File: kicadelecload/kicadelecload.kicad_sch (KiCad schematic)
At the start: 9 parts, among them Q1 IRF540N, Q2 IRF540N, Q3 IRF540N, Q4 IRF540N, U1 ESP32-S2-DEVKITC-1, U2 LM358, U3 TL431D

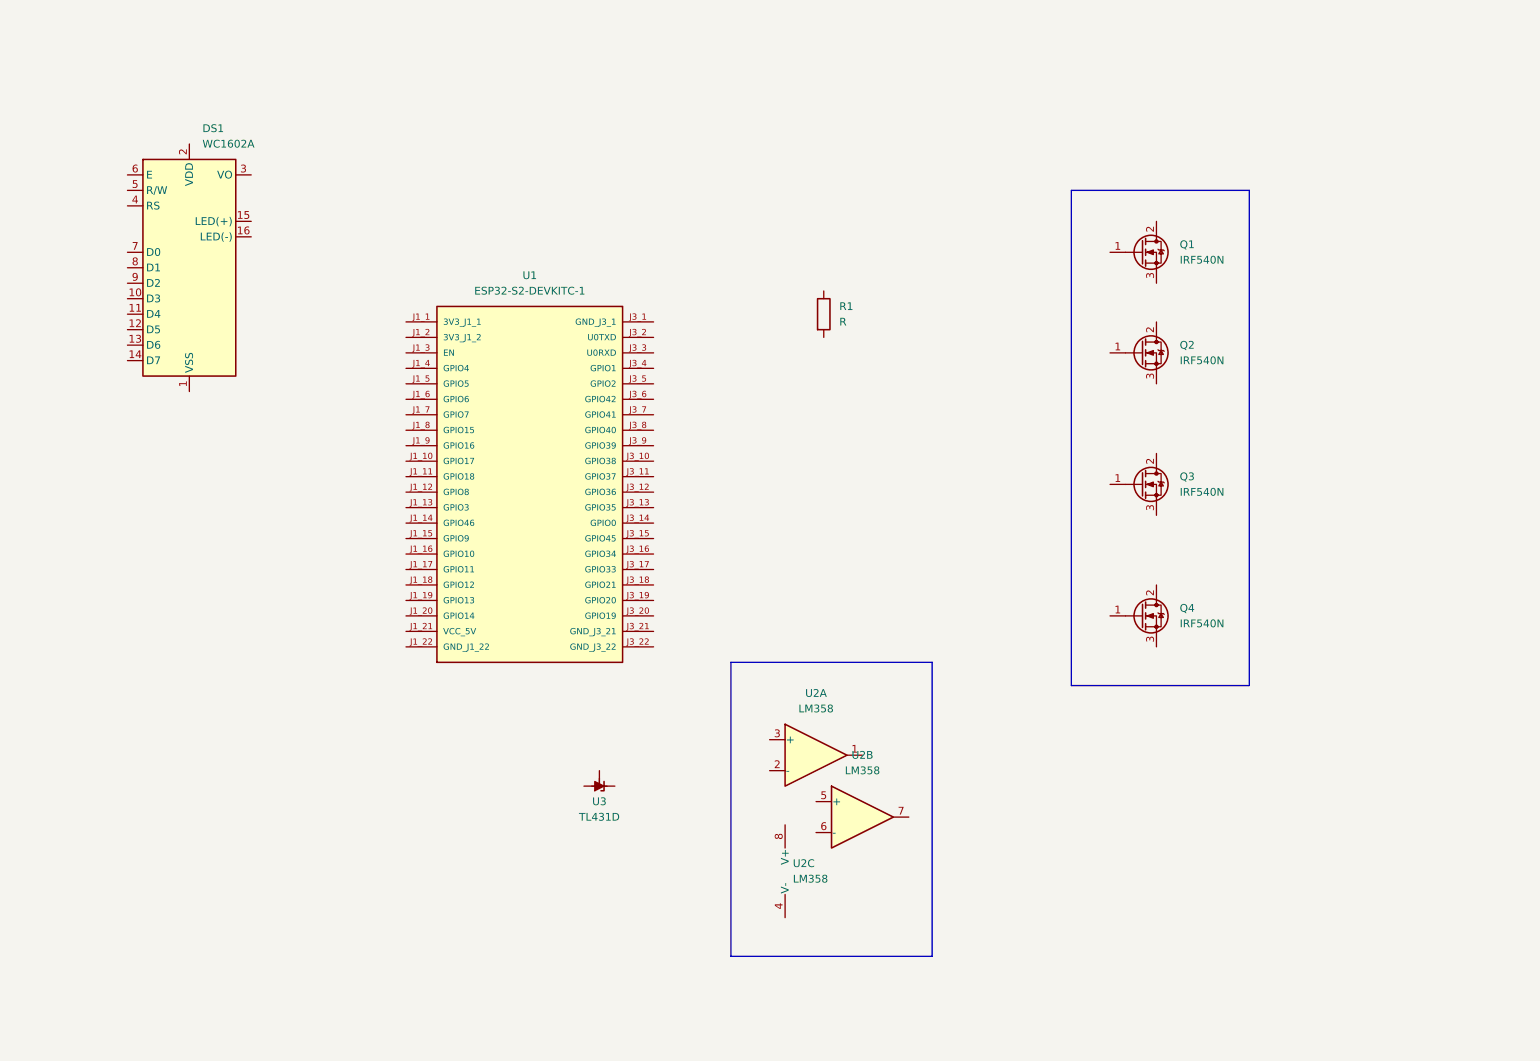
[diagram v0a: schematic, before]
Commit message: schéma electrique V1 commit 1
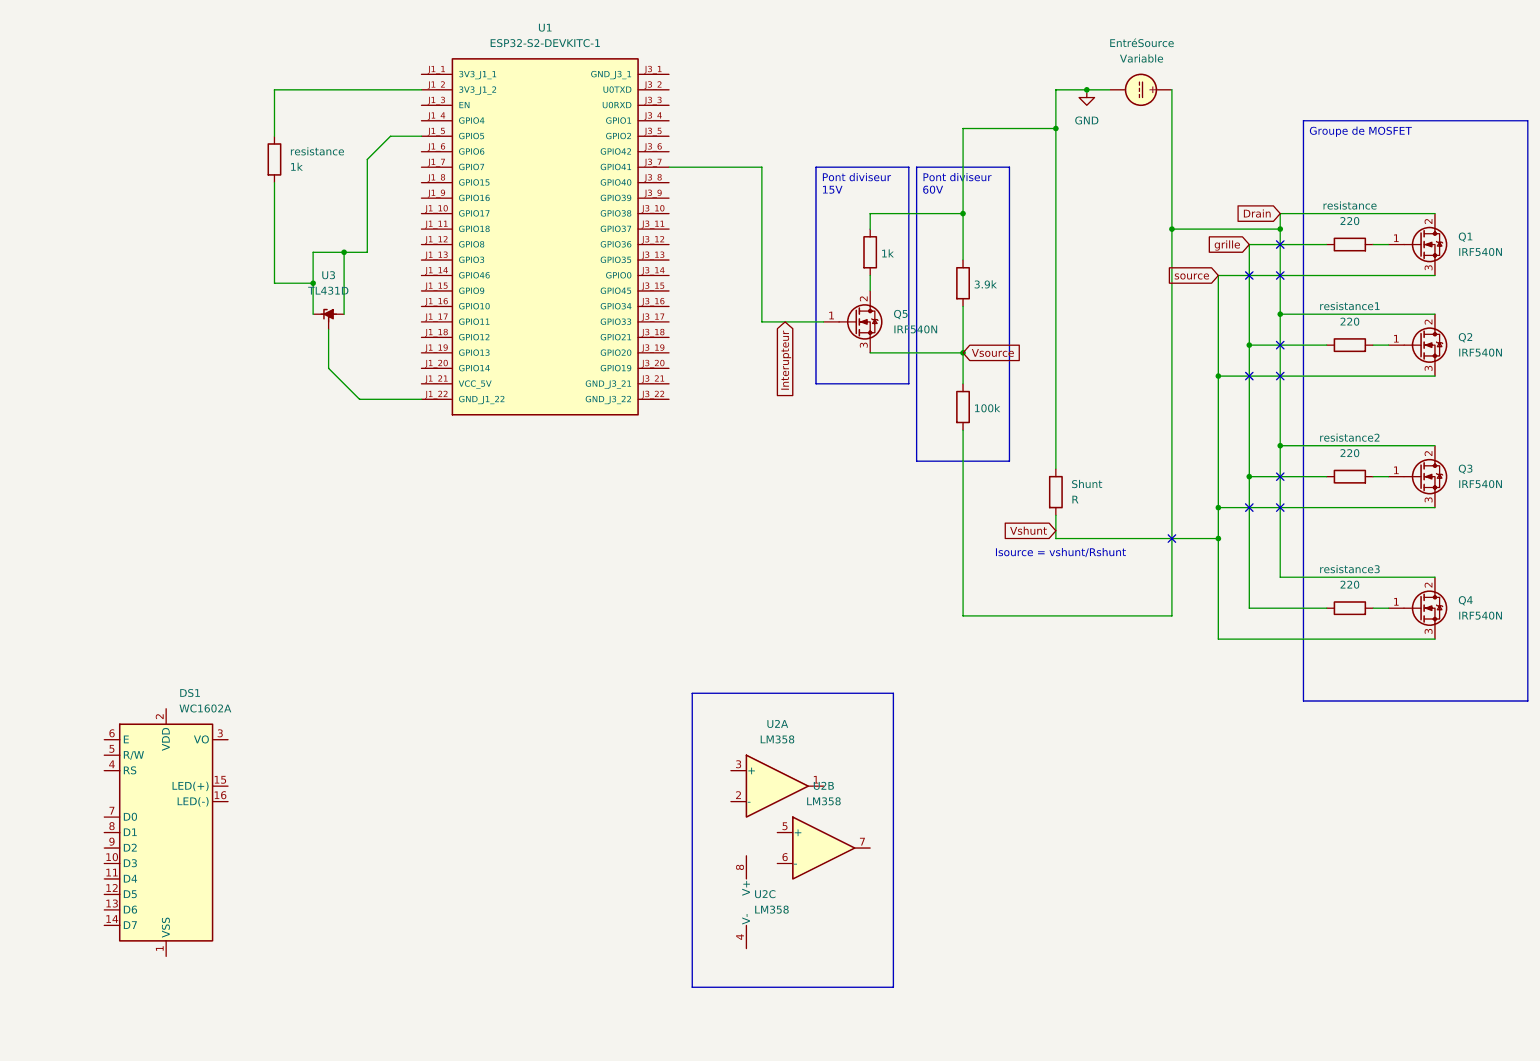
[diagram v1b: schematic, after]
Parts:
- added EntréSource: Variable, symbol Simulation_SPICE:VDC
- added Q5: IRF540N, Package_TO_SOT_THT:TO-220-3_Vertical, symbol Transistor_FET:IRF540N
- added resistance, resistance5: 1k, symbol Device:R
- added resistance, resistance1, resistance2, resistance3: 220, symbol Device:R
- added resistance4: 3.9k, symbol Device:R
- added resistance7: 100k, symbol Device:R
- renumbered R1 to Shunt
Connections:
- net at Q2.1 (G): now also resistance1.2
- net Drain: now reaches Q2.2 (D)
- net Drain: now also Q1.2 (D), Q3.2 (D), Q4.2 (D), EntréSource.1, resistance7.2
- net Vshunt: now reaches Q2.3 (S)
- net Vshunt: now also Q1.3 (S), Q3.3 (S), Q4.3 (S), Shunt.2
- net GND: now reaches Shunt.1
- net GND: now also EntréSource.2, resistance4.1, resistance5.1
- net at Q1.1 (G): now also resistance.2
- net at Q4.1 (G): now also resistance3.2
- net at Q3.1 (G): now also resistance2.2
- net at U3.1 (K): now also U1.J1_5 (GPIO5), U3.2 (A), U3.3 (A), U3.6 (A), U3.7 (A), resistance.2
- net at U3.8 (REF): now also U1.J1_22 (GND_J1_22)
- net at U1.J1_2 (3V3_J1_2): now also resistance.1
- net Interupteur: now reaches U1.J3_7 (GPIO41)
- net Interupteur: now also Q5.1 (G)
- new net: Q5.2 (D), resistance5.2
- new net Vsource: Q5.3 (S), resistance4.2, resistance7.1
- new net grille: resistance.1, resistance1.1, resistance2.1, resistance3.1
- no-connect marks 0 -> 10
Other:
- note added: "Isource = vshunt/Rshunt"
- moved on the sheet: DS1, Q1, Q2, Q3, Q4, Shunt, U1, U2A, U2B, U2C, U3

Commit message: schema electrique V1 commit 2
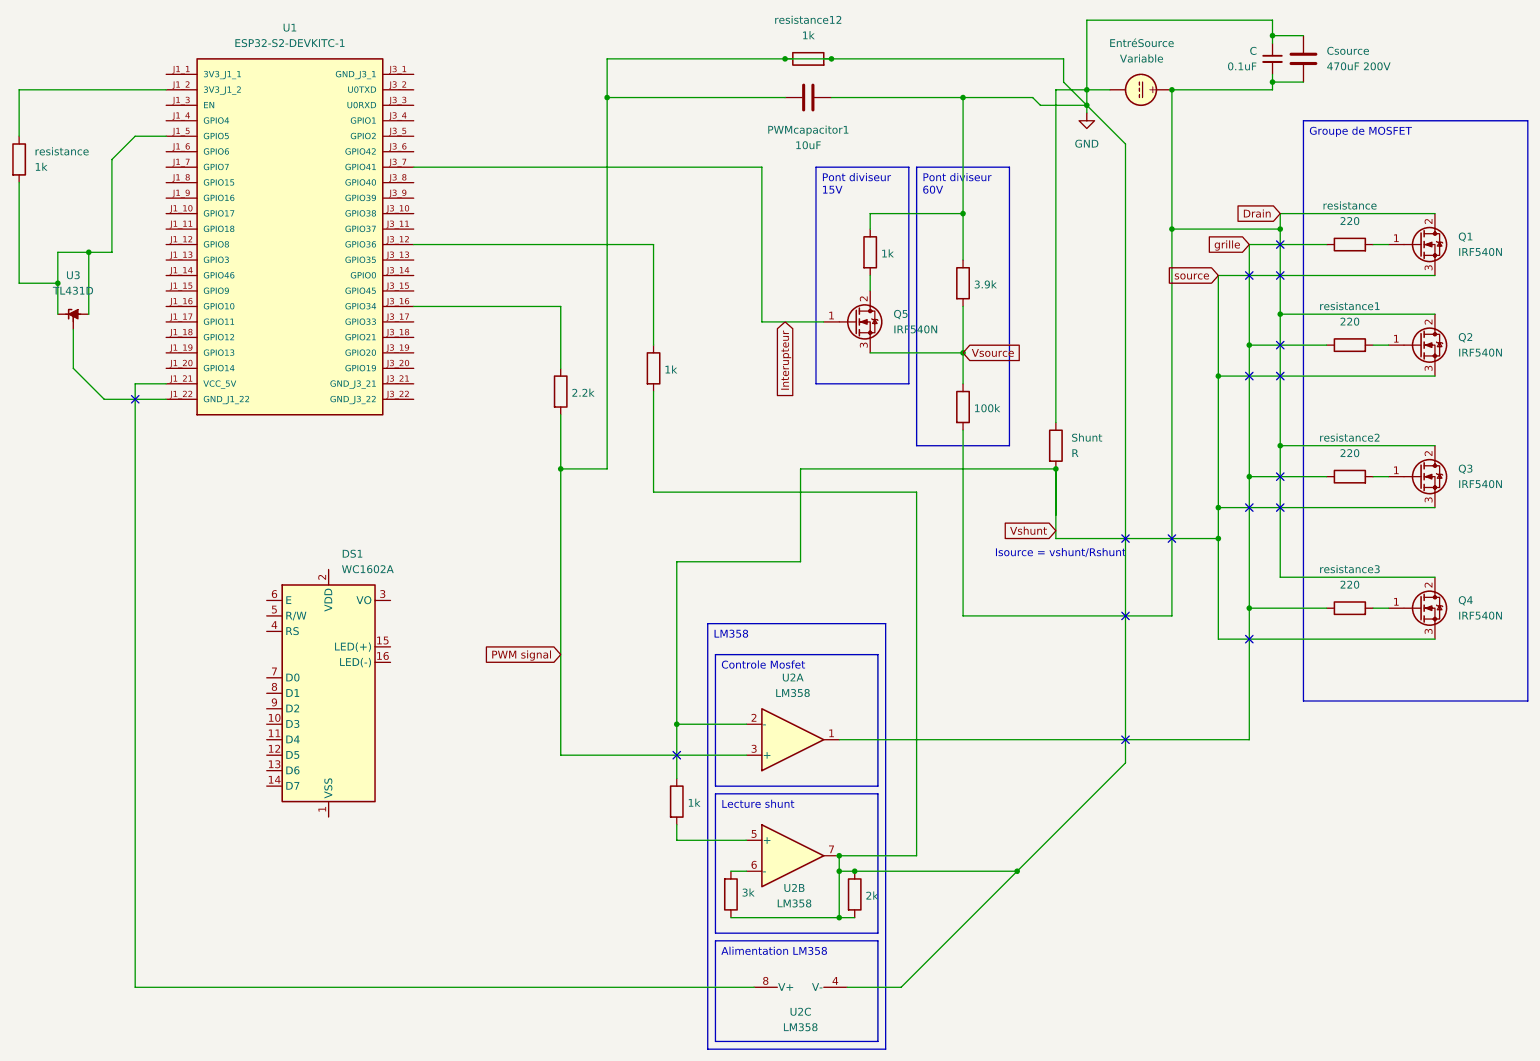
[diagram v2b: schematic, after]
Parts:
- added C: 0.1uF, symbol Device:C_Small
- added Csource: 470uF 200V, symbol Device:C
- added PWMcapacitor1: 10uF, symbol Device:C
- added resistance10, resistance12, resistance6: 1k, symbol Device:R
- added resistance11: 2.2k, symbol Device:R
- added resistance8: 3k, symbol Device:R
- added resistance9: 2k, symbol Device:R
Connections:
- net Drain: now also C.2, Csource.2
- net GND: now also U2.3 (+), U2.4 (V-), U2.7, C.1, Csource.1, PWMcapacitor1.1, PWMcapacitor1.2, resistance10.2, resistance11.2, resistance12.1, resistance12.2, resistance8.1, resistance9.1, resistance9.2
- net Vshunt: now also U2.2 (-), resistance6.1
- net grille: now also U2.1
- net at U2.5 (+): now also resistance6.2
- net at U2.6 (-): now also resistance8.2
- net at U2.8 (V+): now also U1.J1_21 (VCC_5V)
- net at U1.J3_12 (GPIO36): now also resistance10.1
- net at U1.J3_16 (GPIO34): now also resistance11.1
- no-connect marks 10 -> 16
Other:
- moved on the sheet: DS1, Shunt, U1, U2A, U2B, U2C, U3, resistance
